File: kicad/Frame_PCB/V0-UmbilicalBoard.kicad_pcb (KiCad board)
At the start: 2 copper layers, 122 x 37 mm, 16 parts, among them J1 Conn_02x08_Odd_Even, J10 Neopixel Strip 1, J11 Neopixel Strip 1, J12 Neopixel Out, J2 Motor, J3 Hotend Fan, J4 Part Cooling Fan, J5 Heater, J6 Thermistor, J7 X-Endstop, J8 Chamber Thermistor, J9 Neopixel (from controller)

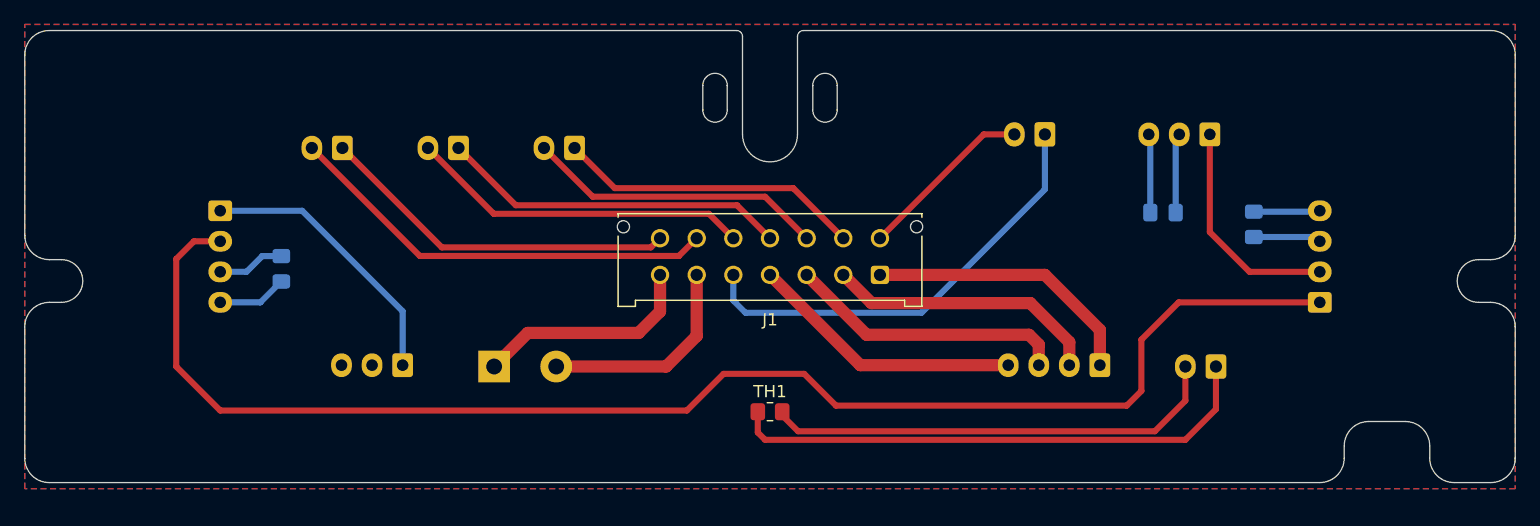
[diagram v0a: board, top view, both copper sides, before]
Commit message: v0 2020
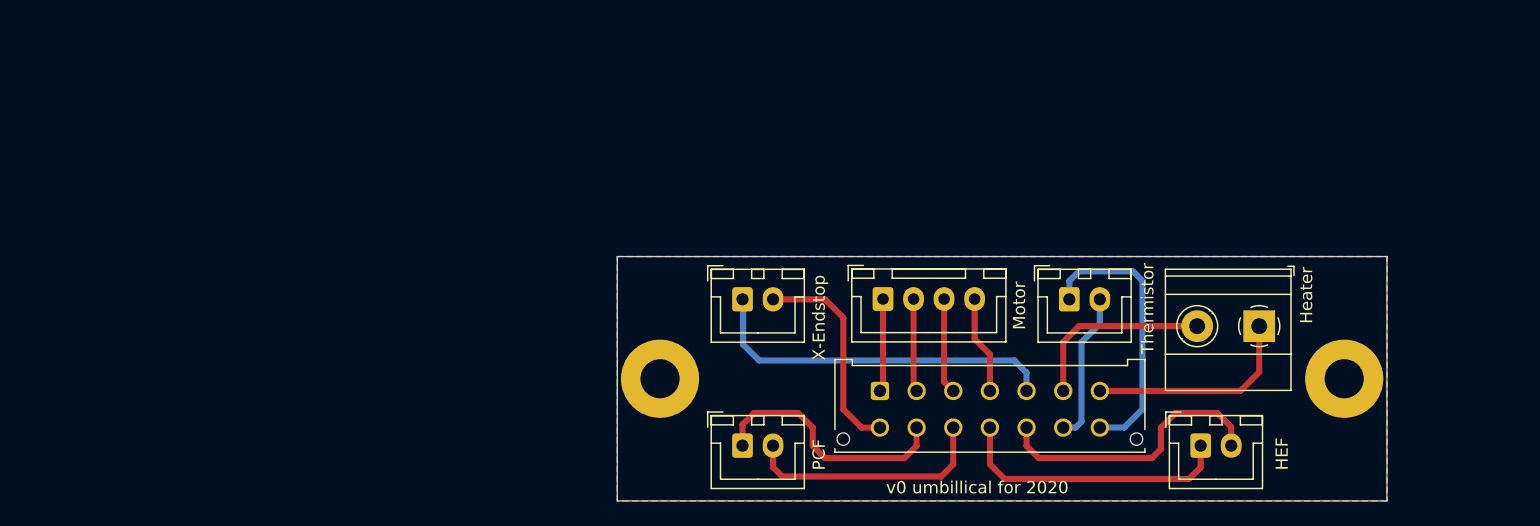
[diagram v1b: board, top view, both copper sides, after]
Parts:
- removed C1, C2, C3: C, Capacitor_SMD:C_0805_2012Metric_Pad1.18x1.45mm_HandSolder
- removed J10, J11: Neopixel Strip 1, Connector_JST:JST_XH_B4B-XH-A_1x04_P2.50mm_Vertical
- removed J12: Neopixel Out, Connector_JST:JST_XH_B3B-XH-A_1x03_P2.50mm_Vertical
- removed J8: Chamber Thermistor, Connector_JST:JST_XH_B2B-XH-A_1x02_P2.50mm_Vertical
- removed J9: Neopixel (from controller), Connector_JST:JST_XH_B3B-XH-A_1x03_P2.50mm_Vertical
- removed TH1: Thermistor, Resistor_SMD:R_0805_2012Metric_Pad1.20x1.40mm_HandSolder
- added H1: MountingHole_Pad, MountingHole:MountingHole_3.2mm_M3_Pad, F.Cu at (91.0, 110.0)
- added H2: MountingHole_Pad, MountingHole:MountingHole_3.2mm_M3_Pad, F.Cu at (147.0, 110.0)
- J2, J3, J4, J5, J6, J7: moved to F.Cu
- moved J3 65.5 mm to (135.2, 115.5), turned to 0 degrees
- moved J5 62.7 mm to (140.0, 105.7), turned to 180 degrees
- moved J6 60.8 mm to (124.5, 103.5), turned to 0 degrees
- moved J7 28.2 mm to (97.8, 103.5), turned to 0 degrees
- moved J4 28.0 mm to (97.8, 115.5), turned to 0 degrees
- moved J2 18.6 mm to (109.2, 103.5), turned to 0 degrees
- moved J1 9.50 mm to (109.0, 111.0), turned to 0 degrees
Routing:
- net DataIn2: track 116.4 -> 0.00 mm
- net Net-(J8-Pad1): track 44.0 -> 0.00 mm
- net Net-(J8-Pad2): track 37.7 -> 0.00 mm
- net Net-(J1-Pin_13): track 35.8 -> 12.3 mm
- net DataIn3: track 22.8 -> 0.00 mm
- net Data: track 18.3 -> 0.00 mm
- net 5V: track 17.6 -> 0.00 mm
- net GND: track 17.6 -> 0.00 mm
- net /B1: track 23.1 -> 7.84 mm
- net /A1: track 22.8 -> 7.63 mm
- net /A2: track 22.7 -> 7.63 mm
- net /B2: track 22.6 -> 8.04 mm
- net Net-(J1-Pin_5): track 36.7 -> 29.4 mm
- net Net-(J1-Pin_14): track 29.7 -> 22.8 mm
- net /Hotend_Fan-: track 28.6 -> 22.9 mm
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- added copper zone on F.Cu, net GND
- removed copper zone on F.Cu, net 5V
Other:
- board size 122 x 37 mm -> 63 x 20 mm
- board text added: "HEF"
- board text added: "Motor"
- board text added: "PCF"
- board text added: "Thermistor"
- board text added: "v0 umbillical for 2020"
- board text removed: "+ -"
- board text removed: "- +"
- board text removed: "Chamber Thermistor"
- board text removed: "Gnd +5V In Out Neopixel Strip 1"
- board text removed: "Gnd +5V In Out Neopixel Strip 2"
- board text removed: "Hotend"
- board text removed: "Hotend Thermistor"
- board text removed: "Motor A1 A2 B1 B2"
- board text removed: "Neopixel (to controller) Data +5 Gnd"
- board text removed: "Neopixel Strip 3 In +5V Gnd"
- board text removed: "Part Cooling"
- board text removed: "V0 Umbilical Breakout Board Rev A.1 - 5/14/22 T. Abraham"
